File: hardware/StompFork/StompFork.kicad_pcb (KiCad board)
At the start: 2 copper layers, 100.3 x 50.8 mm, 34 parts, among them J1 Line-Level Input, J2 Direct Output, J3 Stompbox Output 1, J4 Stompbox Output 2, J5 Power, U1 TL074

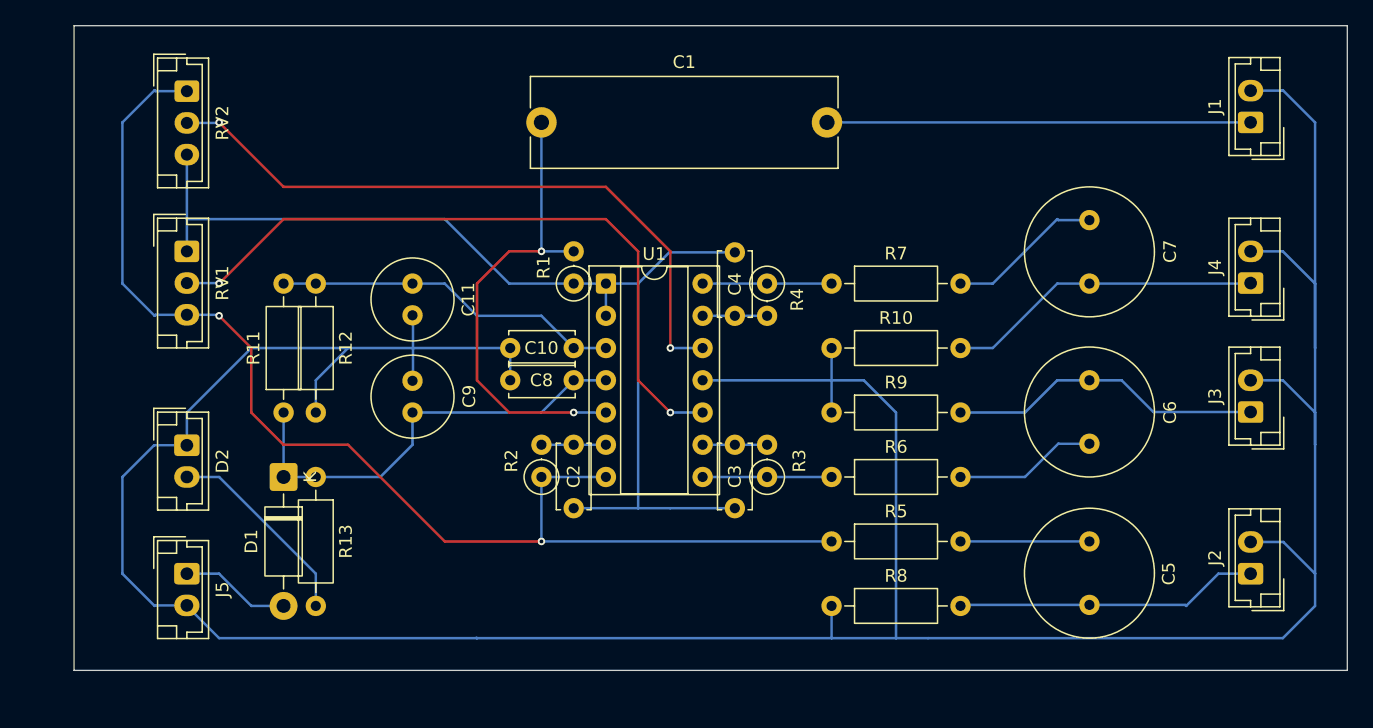
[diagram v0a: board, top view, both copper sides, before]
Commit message: Update PCB
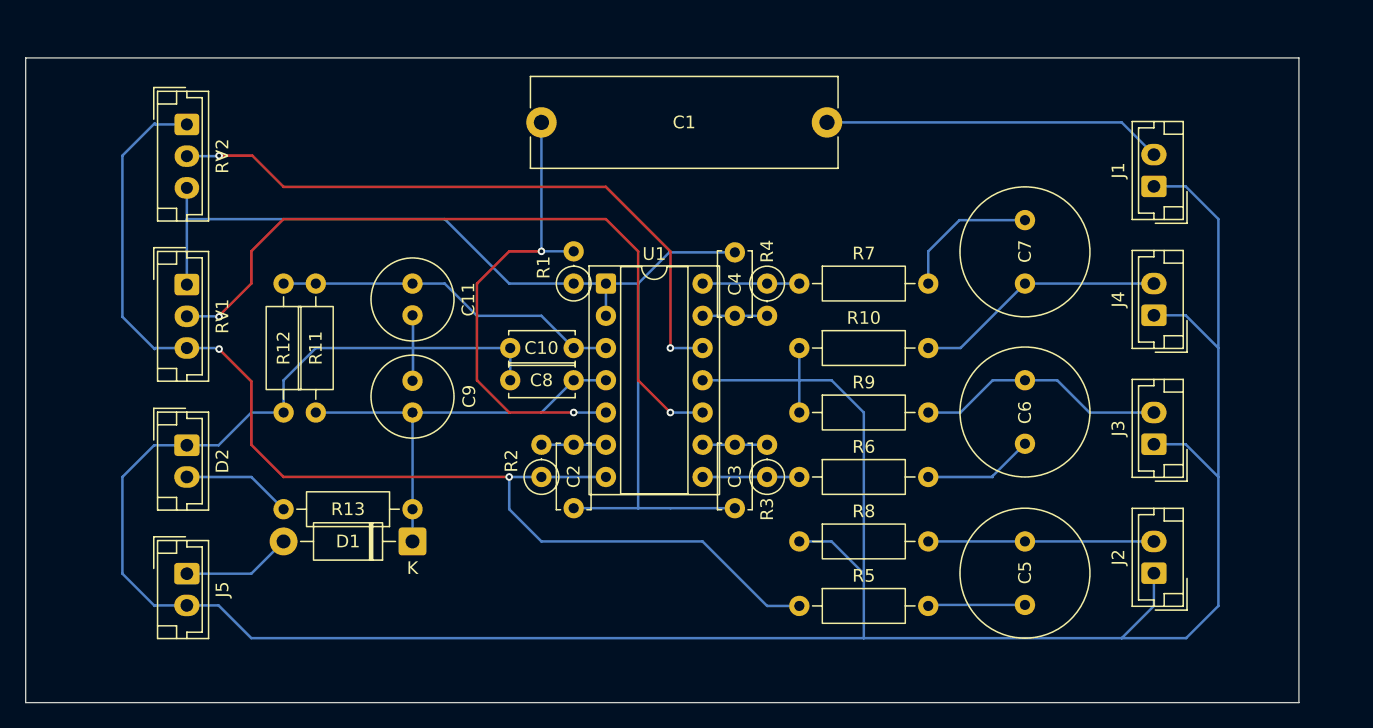
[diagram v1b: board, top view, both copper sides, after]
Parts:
- moved D1 11.4 mm to (127.0, 116.8), turned to 180 degrees
- moved J1 9.14 mm to (185.4, 88.9)
- moved J3 8.03 mm to (185.4, 109.2)
- moved J4 8.03 mm to (185.4, 99.0)
- moved R13 8.03 mm to (127.0, 114.3), turned to 180 degrees
- moved J2 7.62 mm to (185.4, 119.3)
- moved C5 7.13 mm to (175.3, 121.8), turned to 90 degrees
- moved R5 5.68 mm to (157.5, 121.9)
- moved R8 5.68 mm to (157.5, 116.8)
- moved C6 5.08 mm to (175.3, 109.1)
- moved C7 5.08 mm to (175.3, 91.5)
- moved RV2 2.62 mm to (109.2, 84.0)
- moved RV1 2.62 mm to (109.2, 96.6)
- moved R10 2.54 mm to (157.5, 101.6)
- moved R6 2.54 mm to (157.5, 111.8)
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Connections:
- J1 pad 1: Net-(J1-T) -> GND
- J1 pad 2: GND -> Net-(J1-T)
- J2 pad 1: Net-(J2-T) -> GND
- J2 pad 2: GND -> Net-(J2-T)
- J3 pad 1: Net-(J3-T) -> GND
- J3 pad 2: GND -> Net-(J3-T)
- J4 pad 1: Net-(J4-T) -> GND
- J4 pad 2: GND -> Net-(J4-T)
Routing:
- net GND: track 266.9 -> 239.0 mm
- net Net-(D2-A): track 15.9 -> 8.67 mm
- net Net-(J1-T): track 33.4 -> 26.8 mm
- net Net-(J2-T): track 24.0 -> 17.8 mm
- net Net-(J3-T): track 24.9 -> 19.9 mm
- net Net-(J4-T): track 25.0 -> 19.9 mm
- net Net-(R2-Pad1): track 96.4 -> 93.7 mm
- net Net-(U1C-+): track 55.1 -> 57.7 mm
- net Net-(R4-Pad1): track 10.2 -> 7.62 mm
- net Net-(R3-Pad1): track 10.2 -> 7.62 mm
- net Net-(C6-Pad1): track 11.2 -> 8.75 mm
- net Net-(C5-Pad1): track 10.2 -> 7.77 mm
- net Net-(C7-Pad1): track 12.3 -> 11.2 mm
- net Net-(U1D-+): track 52.5 -> 51.4 mm
- net VCC: track 35.1 -> 34.1 mm
